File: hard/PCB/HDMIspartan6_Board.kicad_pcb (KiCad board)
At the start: 2 copper layers, 58.5 x 99 mm, 249 parts, among them J1 CONN_02X09, J2 B6B-PH-K-S(LF)(SN), J3 HDMI_A, P1 CONN_02X20, P2 CONN_02X03, P3 CONN_01X03, P4 CONN_02X05, P5 CONN_02X05, U1 XC6SLX9-2TQG144C, U2 TPS62133RGTR, U3 ZLDO1117G33TA, U4 ZLDO1117G12TA, U5 MAX5864, U6 S25FL064LABMFI013, U7 ATMEGA32U4-A

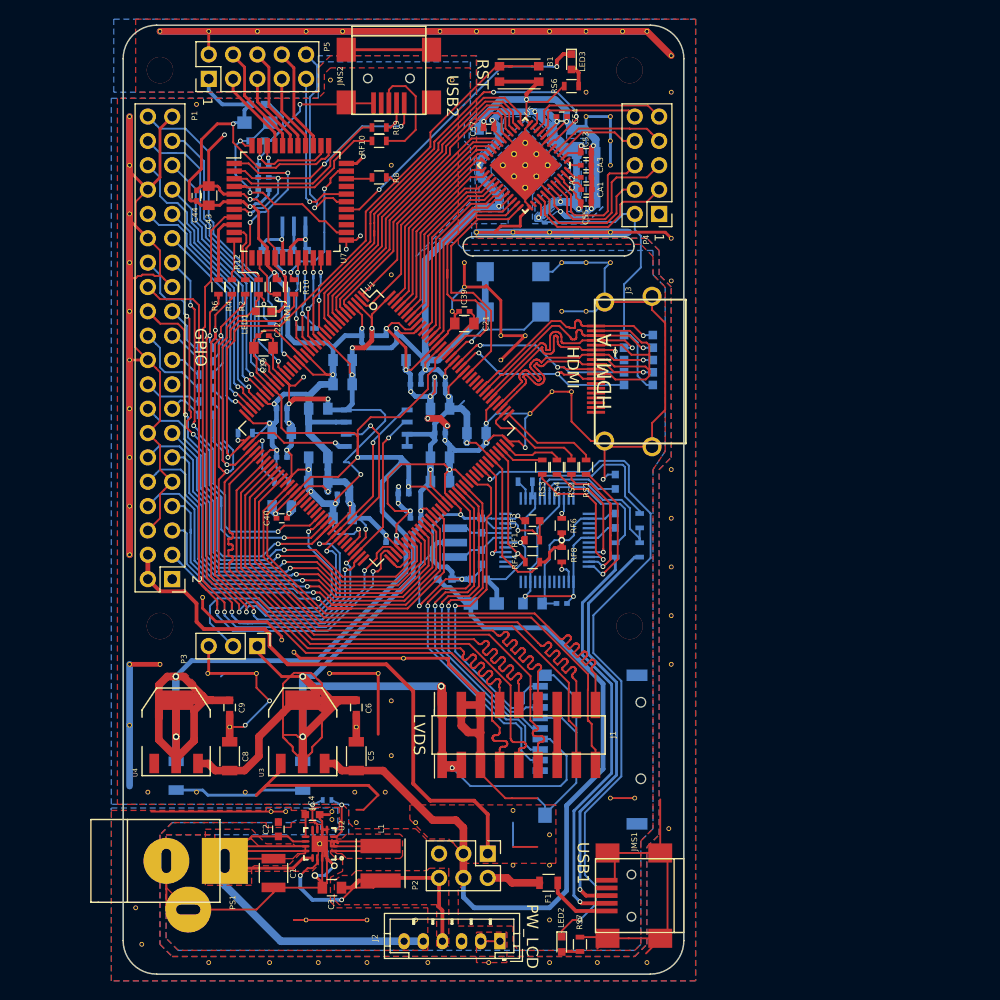
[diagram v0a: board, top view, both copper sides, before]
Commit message: SilkS 2
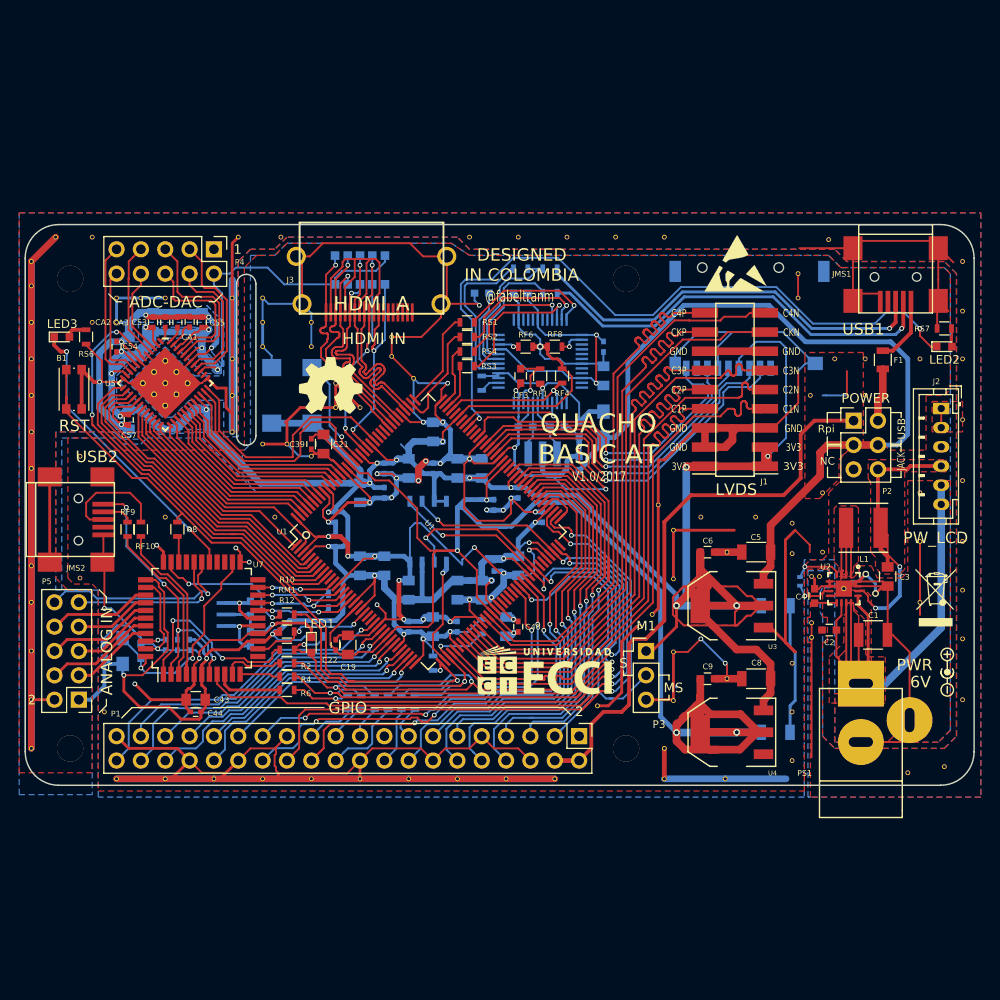
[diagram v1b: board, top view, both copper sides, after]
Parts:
- added G***: LOGO, Project:uECCI_Logo_silkS, F.Cu at (152.6, 119.8)
- added G***: LOGO, Project:Logo_silk_polarity_center_5x1.4mm, F.Cu at (194.6, 120.1)
- added REF***: OSHW-Symbol_6.7x6mm_SilkScreen, Symbols:OSHW-Symbol_6.7x6mm_SilkScreen, F.Cu at (130.3, 90.2)
- added REF***: ESD-Logo_6.6x6mm_SilkScreen, Symbols:ESD-Logo_6.6x6mm_SilkScreen, F.Cu at (172.6, 77.4)
- added REF***: WEEE-Logo_4.2x6mm_SilkScreen, Symbols:WEEE-Logo_4.2x6mm_SilkScreen, F.Cu at (193.4, 112.3)
- moved TH27 85.8 mm to (194.3, 129.9), turned to 90 degrees
- moved TH22 83.3 mm to (196.2, 123.0), turned to 90 degrees
- moved TH1 81.8 mm to (190.5, 130.6), turned to 270 degrees
- moved TH24 80.2 mm to (196.2, 77.2), turned to 90 degrees
- moved TH29 79.8 mm to (196.2, 116.6), turned to 90 degrees
- moved TH39 77.9 mm to (196.2, 82.4), turned to 90 degrees
- moved TH38 77.6 mm to (196.2, 111.5), turned to 90 degrees
- moved TH109 76.3 mm to (196.2, 87.4), turned to 90 degrees
- moved TH30 76.1 mm to (196.2, 106.4), turned to 90 degrees
- moved TH93 76.0 mm to (99.1, 128.0), turned to 90 degrees
- moved TH108 75.2 mm to (196.2, 93.7), turned to 90 degrees
- moved TH110 75.1 mm to (196.2, 100.1), turned to 90 degrees
- moved RS7 74.7 mm to (194.3, 84.2), turned to 0 degrees
- moved LED2 74.0 mm to (194.3, 86.1), turned to 0 degrees
- moved PS1 73.5 mm to (185.6, 127.4), turned to 90 degrees
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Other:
- board size 58.5 x 99 mm -> 99 x 58.5 mm
- board text added: "-"
- board text added: "3V3"
- board text added: "5V"
- board text added: "6V"
- board text added: "@fabeltranm"
- board text added: "A00"
- board text added: "A01"
- board text added: "A04"
- board text added: "A05"
- board text added: "A06"
- board text added: "A07"
- board text added: "A11"
- board text added: "A12"
- board text added: "ADC-DAC"
- board text added: "ANALOG IN"
- board text added: "C1N"
- board text added: "C1P"
- board text added: "C2N"
- board text added: "C2P"
- board text added: "C3N"
- board text added: "C3P"
- board text added: "C4N"
- board text added: "C4P"
- board text added: "CKN"
- board text added: "CKP"
- board text added: "CS"
- board text added: "DESIGNED IN COLOMBIA"
- board text added: "G04"
- board text added: "G05"
- board text added: "G06"
- board text added: "G08"
- board text added: "G12"
- board text added: "G13"
- board text added: "G16"
- board text added: "G17"
- board text added: "G18"
- board text added: "G19"
- board text added: "G20"
- board text added: "G21"
- board text added: "G23"
- board text added: "G26"
- board text added: "G27"
- board text added: "GND"
- board text added: "HDMI IN"
- board text added: "IA+"
- board text added: "IA-"
- board text added: "ID+"
- board text added: "ID-"
- board text added: "JACK"
- board text added: "M1"
- board text added: "MISO"
- board text added: "MOSI"
- board text added: "MS"
- board text added: "NC"
- board text added: "POWER"
- board text added: "PWR"
- board text added: "QA+"
- board text added: "QA-"
- board text added: "QD+"
- board text added: "QD-"
- board text added: "QUACHO BASIC AT"
- board text added: "RXD"
- board text added: "Rpi"
- board text added: "S"
- board text added: "SCK"
- board text added: "SCL"
- board text added: "SDA"
- board text added: "TXD"
- board text added: "U1"
- board text added: "U5"
- board text added: "USB"
- board text added: "V1.0/2017"
- board text added: "VCC"
- board text removed: "HDMI"

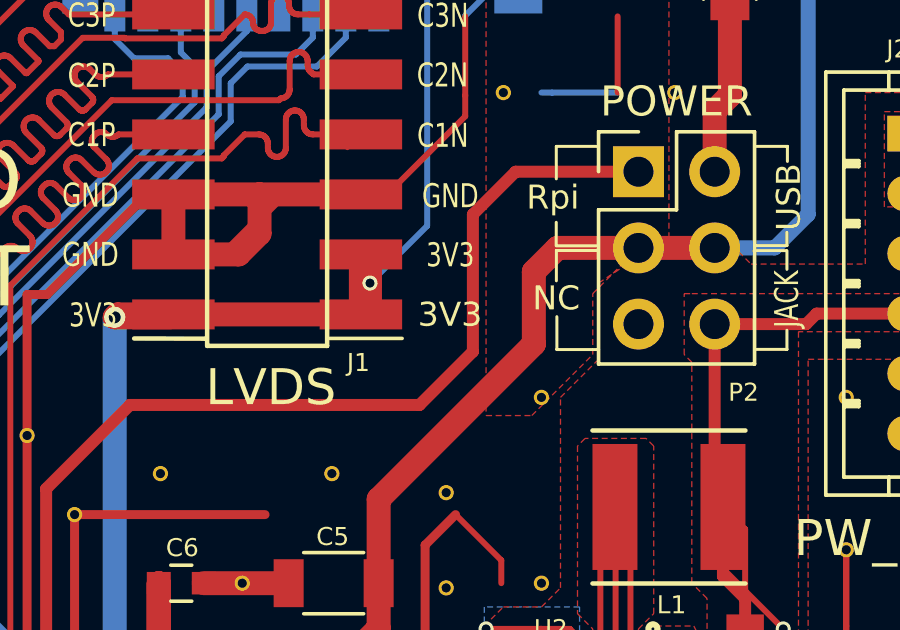
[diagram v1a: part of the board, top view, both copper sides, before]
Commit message: SilkS 2.1
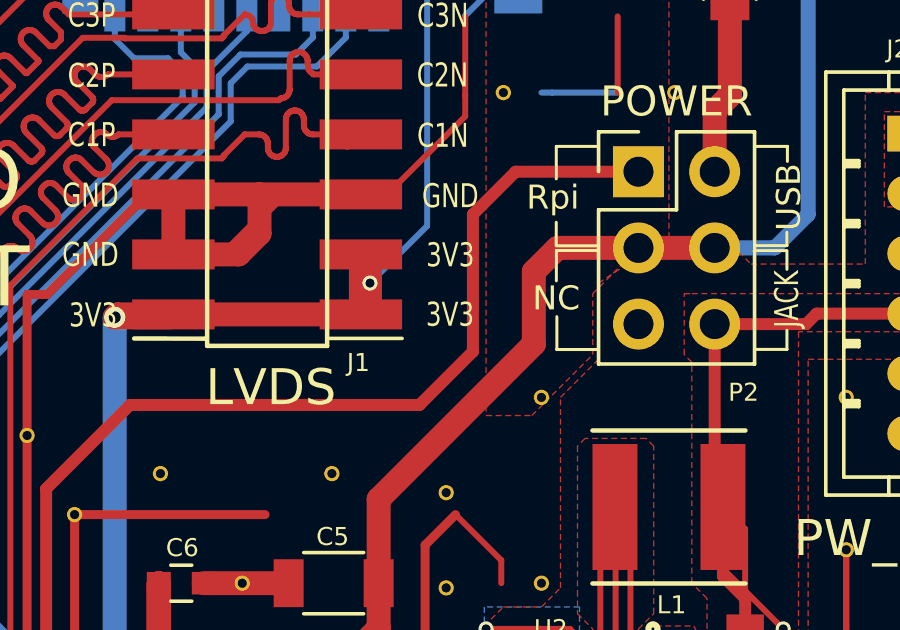
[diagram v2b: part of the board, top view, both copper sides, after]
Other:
- board text added: "ZONA SUGERIDA PARA EL ARTE INSPIRADO EN K3os"
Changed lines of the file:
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@@
     (links 618)
     (no_connects 0)
-    (area 97.81096 66.44882 256.244758 137.523071)
+    (area 98.363959 73.303879 197.513961 131.953881)
     (thickness 1.6)
-    (drawings 165)
+    (drawings 172)
     (tracks 4419)
     (zones 0)
@@
     (31 B.Cu signal hide)
     (32 B.Adhes user)
-    (33 F.Adhes user)
+    (33 F.Adhes user hide)
     (34 B.Paste user)
-    (35 F.Paste user)
+    (35 F.Paste user hide)
     (36 B.SilkS user)
-    (37 F.SilkS user)
+    (37 F.SilkS user hide)
     (38 B.Mask user)
     (39 F.Mask user)
@@
     (aux_axis_origin 20 90)
     (grid_origin 108.037 156.932)
-    (visible_elements 7FFEFFFF)
+    (visible_elements 7FFEBFDF)
     (pcbplotparams
       (layerselection 0x013ff_80000001)
@@
       (xy 1.530863 -2.420002) (xy 1.583231 -2.473048) (xy 2.125049 -3.022233) (xy 2.12443 -2.935152)) (layer F.SilkS) (width 0.01))
   )
+  (gr_text "ZONA SUGERIDA \nPARA EL ARTE\nINSPIRADO EN K3os" (at 179.48974 105.43604) (layer Dwgs.User)
+    (effects (font (size 0.8 1.5) (thickness 0.2)))
+  )
+  (gr_line (start 161.08744 112.99254) (end 161.08744 92.10104) (angle 90) (layer Dwgs.User) (width 0.1))
+  (gr_line (start 165.79914 112.99254) (end 161.08744 112.99254) (angle 90) (layer Dwgs.User) (width 0.1))
+  (gr_line (start 165.79914 133.79514) (end 165.79914 112.99254) (angle 90) (layer Dwgs.User) (width 0.1))
+  (gr_line (start 198.69214 133.79514) (end 165.79914 133.79514) (angle 90) (layer Dwgs.User) (width 0.1))
+  (gr_line (start 198.69214 91.65654) (end 198.69214 133.79514) (angle 90) (layer Dwgs.User) (width 0.1))
+  (gr_line (start 161.35414 91.65654) (end 198.69214 91.65654) (angle 90) (layer Dwgs.User) (width 0.1))
   (gr_text C1N (at 178.34166 92.63952) (layer F.SilkS)
     (effects (font (size 0.8 0.6) (thickness 0.12)))
@@
   )
   (gr_text 3V3 (at 178.58296 98.60344) (layer F.SilkS)
-    (effects (font (size 0.8 0.8) (thickness 0.12)))
+    (effects (font (size 0.8 0.6) (thickness 0.12)))
   )
   (gr_text A00 (at 105.53256 120.41442 90) (layer B.SilkS)
